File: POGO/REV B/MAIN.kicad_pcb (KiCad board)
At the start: 2 copper layers, 22.9 x 11.4 mm, 2 parts, among them P1 4 PIN POGO, P2 TE 1X4

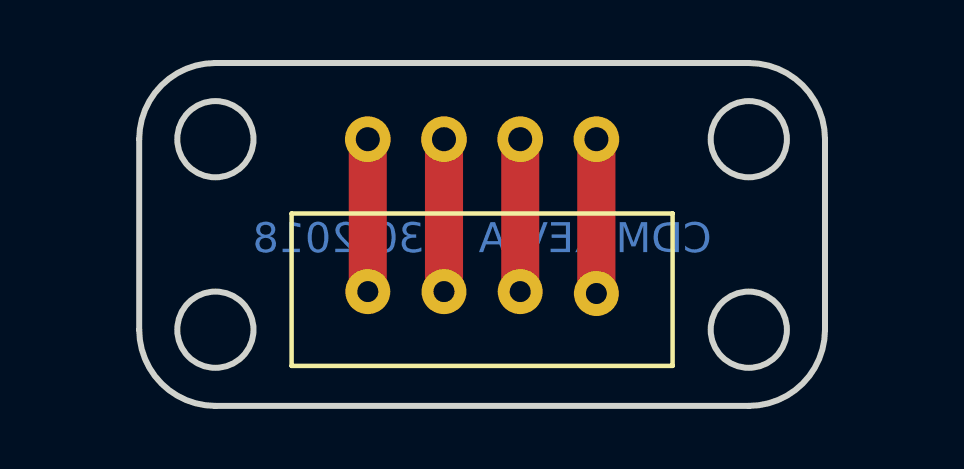
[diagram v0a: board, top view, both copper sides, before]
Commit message: REV B Pogo
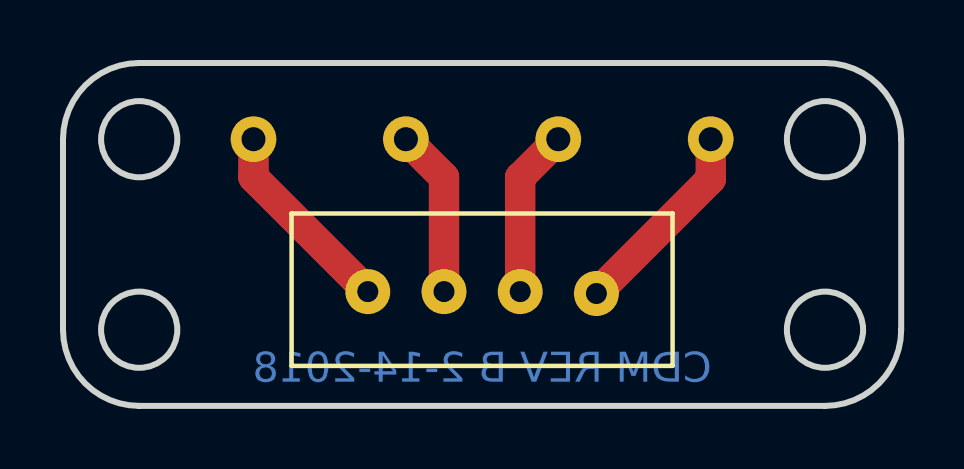
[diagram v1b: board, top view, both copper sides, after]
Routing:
- net Net-(P1-Pad4): track 5.14 -> 6.72 mm
- net Net-(P1-Pad1): track 5.08 -> 6.66 mm
- net Net-(P1-Pad3): track 5.08 -> 5.61 mm
- net Net-(P1-Pad2): track 5.08 -> 5.61 mm
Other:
- board size 22.9 x 11.4 mm -> 27.9 x 11.4 mm
- board text added: "CDM REV B 2-14-2018"
- board text removed: "CDM REV A 1-30-2018"
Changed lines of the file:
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@@
 (kicad_pcb (version 4) (host pcbnew 4.0.5+dfsg1-4)
   (general
-    (links 0)
+    (links 4)
     (no_connects 0)
-    (area 144.679999 88.799999 167.740001 100.430001)
+    (area 74.282299 87.9853 170.280001 102.446103)
     (thickness 1.6)
     (drawings 14)
-    (tracks 19)
+    (tracks 23)
     (zones 0)
     (modules 2)
@@
     (add_net "Net-(P1-Pad4)")
   )
-  (module "MOD:4 PIN POGO" (layer F.Cu)
-    (at 156.21 91.44)
-    (fp_text reference P1 (at 0 0.5) (layer F.SilkS) hide
-      (effects (font (size 1 1) (thickness 0.15)))
-    )
-    (fp_text value "4 PIN POGO" (at 0 -2.54) (layer F.Fab)
-      (effects (font (size 1 1) (thickness 0.15)))
-    )
-    (pad 1 thru_hole circle (at -3.81 0) (size 1.524 1.524) (drill 0.8) (layers *.Cu *.Mask)
-      (net 1 "Net-(P1-Pad1)"))
-    (pad 2 thru_hole circle (at -1.27 0) (size 1.524 1.524) (drill 0.8) (layers *.Cu *.Mask)
-      (net 2 "Net-(P1-Pad2)"))
-    (pad 3 thru_hole circle (at 1.27 0) (size 1.524 1.524) (drill 0.8) (layers *.Cu *.Mask)
-      (net 3 "Net-(P1-Pad3)"))
-    (pad 4 thru_hole circle (at 3.81 0) (size 1.524 1.524) (drill 0.8) (layers *.Cu *.Mask)
-      (net 4 "Net-(P1-Pad4)"))
-  )
   (module MOD:TE1X4_5-103669-3 (layer F.Cu)
     (at 154.94 93.9165)
@@
       (net 4 "Net-(P1-Pad4)"))
   )
-  (gr_text "TOLEDO ROCKETRY CLUB" (at 156.21 93.472) (layer B.SilkS)
+  (module "MOD:4 PIN POGO" (layer F.Cu)
+    (at 156.21 91.44)
+    (fp_text reference P1 (at 1.27 0.5) (layer F.SilkS) hide
+      (effects (font (size 1 1) (thickness 0.15)))
+    )
+    (fp_text value "4 PIN POGO" (at 0 -2.54) (layer F.Fab)
+      (effects (font (size 1 1) (thickness 0.15)))
+    )
+    (pad 1 thru_hole circle (at -7.62 0) (size 1.524 1.524) (drill 0.8) (layers *.Cu *.Mask)
+      (net 1 "Net-(P1-Pad1)"))
+    (pad 2 thru_hole circle (at -2.54 0) (size 1.524 1.524) (drill 0.8) (layers *.Cu *.Mask)
+      (net 2 "Net-(P1-Pad2)"))
+    (pad 3 thru_hole circle (at 2.54 0) (size 1.524 1.524) (drill 0.8) (layers *.Cu *.Mask)
+      (net 3 "Net-(P1-Pad3)"))
+    (pad 4 thru_hole circle (at 7.62 0) (size 1.524 1.524) (drill 0.8) (layers *.Cu *.Mask)
+      (net 4 "Net-(P1-Pad4)"))
+  )
+  (gr_text "TOLEDO ROCKETRY CLUB" (at 156.21 93.98) (layer B.SilkS)
     (effects (font (size 1 1) (thickness 0.15)) (justify mirror))
   )
-  (gr_text "CDM REV A 1-30-2018" (at 156.21 94.742) (layer B.Cu)
+  (gr_text "CDM REV B 2-14-2018" (at 156.21 99.06) (layer B.Cu)
     (effects (font (size 1 1) (thickness 0.15)) (justify mirror))
   )
-  (gr_circle (center 147.32 97.79) (end 147.32 96.52) (layer Edge.Cuts) (width 0.2))
-  (gr_circle (center 165.1 97.79) (end 165.1 96.52) (layer Edge.Cuts) (width 0.2))
-  (gr_circle (center 147.32 91.44) (end 147.32 90.17) (layer Edge.Cuts) (width 0.2))
-  (gr_circle (center 165.1 91.44) (end 165.1 90.17) (layer Edge.Cuts) (width 0.2))
-  (gr_arc (start 147.32 91.44) (end 144.78 91.44) (angle 90) (layer Edge.Cuts) (width 0.2))
-  (gr_arc (start 147.32 97.79) (end 147.32 100.33) (angle 90) (layer Edge.Cuts) (width 0.2))
-  (gr_arc (start 165.1 97.79) (end 167.64 97.79) (angle 90) (layer Edge.Cuts) (width 0.2))
-  (gr_arc (start 165.1 91.44) (end 165.1 88.9) (angle 90) (layer Edge.Cuts) (width 0.2))
-  (gr_line (start 144.78 97.79) (end 144.78 91.44) (layer Edge.Cuts) (width 0.2))
-  (gr_line (start 165.1 100.33) (end 147.32 100.33) (layer Edge.Cuts) (width 0.2))
-  (gr_line (start 167.64 91.44) (end 167.64 97.79) (layer Edge.Cuts) (width 0.2))
-  (gr_line (start 147.32 88.9) (end 165.1 88.9) (layer Edge.Cuts) (width 0.2))
+  (gr_circle (center 144.78 97.79) (end 144.78 96.52) (layer Edge.Cuts) (width 0.2))
+  (gr_circle (center 167.64 97.79) (end 167.64 96.52) (layer Edge.Cuts) (width 0.2))
+  (gr_circle (center 144.78 91.44) (end 144.78 90.17) (layer Edge.Cuts) (width 0.2))
+  (gr_circle (center 167.64 91.44) (end 167.64 90.17) (layer Edge.Cuts) (width 0.2))
+  (gr_arc (start 144.78 91.44) (end 142.24 91.44) (angle 90) (layer Edge.Cuts) (width 0.2))
+  (gr_arc (start 144.78 97.79) (end 144.78 100.33) (angle 90) (layer Edge.Cuts) (width 0.2))
+  (gr_arc (start 167.64 97.79) (end 170.18 97.79) (angle 90) (layer Edge.Cuts) (width 0.2))
+  (gr_arc (start 167.64 91.44) (end 167.64 88.9) (angle 90) (layer Edge.Cuts) (width 0.2))
+  (gr_line (start 142.24 97.79) (end 142.24 91.44) (layer Edge.Cuts) (width 0.2))
+  (gr_line (start 167.64 100.33) (end 144.78 100.33) (layer Edge.Cuts) (width 0.2))
+  (gr_line (start 170.18 91.44) (end 170.18 97.79) (layer Edge.Cuts) (width 0.2))
+  (gr_line (start 144.78 88.9) (end 167.64 88.9) (layer Edge.Cuts) (width 0.2))
   (segment (start 95.758 100.838) (end 95.25 101.346) (width 0.7874) (layer In2.Cu) (net 0))
   (segment (start 93.146599 101.671401) (end 93.472 101.346) (width 1.27) (layer In2.Cu) (net 0))
@@
   (segment (start 76.594401 94.882401) (end 76.594401 99.872099) (width 1.27) (layer In2.Cu) (net 0))
   (segment (start 76.594401 99.872099) (end 75.870499 100.596001) (width 1.27) (layer In2.Cu) (net 0))
-  (segment (start 152.4 91.44) (end 152.4 96.52) (width 1.27) (layer F.Cu) (net 1))
-  (segment (start 154.94 91.44) (end 154.94 96.52) (width 1.27) (layer F.Cu) (net 2))
-  (segment (start 157.48 96.52) (end 157.48 91.44) (width 1.27) (layer F.Cu) (net 3))
-  (segment (start 160.02 96.5835) (end 160.02 91.44) (width 1.27) (layer F.Cu) (net 4))
+  (segment (start 148.59 91.44) (end 148.59 92.71) (width 1.016) (layer F.Cu) (net 1))
+  (segment (start 148.59 92.71) (end 152.4 96.52) (width 1.016) (layer F.Cu) (net 1))
+  (segment (start 154.94 96.52) (end 154.94 92.71) (width 1.016) (layer F.Cu) (net 2))
+  (segment (start 154.94 92.71) (end 153.67 91.44) (width 1.016) (layer F.Cu) (net 2))
+  (segment (start 157.48 96.52) (end 157.48 92.71) (width 1.016) (layer F.Cu) (net 3))
+  (segment (start 157.48 92.71) (end 158.75 91.44) (width 1.016) (layer F.Cu) (net 3))
+  (segment (start 163.83 91.44) (end 163.83 92.7735) (width 1.016) (layer F.Cu) (net 4))
+  (segment (start 163.83 92.7735) (end 160.02 96.5835) (width 1.016) (layer F.Cu) (net 4))
 )
